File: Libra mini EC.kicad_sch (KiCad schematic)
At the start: 47 parts, among them J1 USB_C_Receptacle_USB2.0_16P, J3 Conn_01x18, J4 Conn_01x18, U1 STM32G474CBTx, U2 USBLC6-2SC6, U3 TPS7A2033, U4 TPS7A2033, U5 TPS7A2033, Y1 8Mhz 12pF

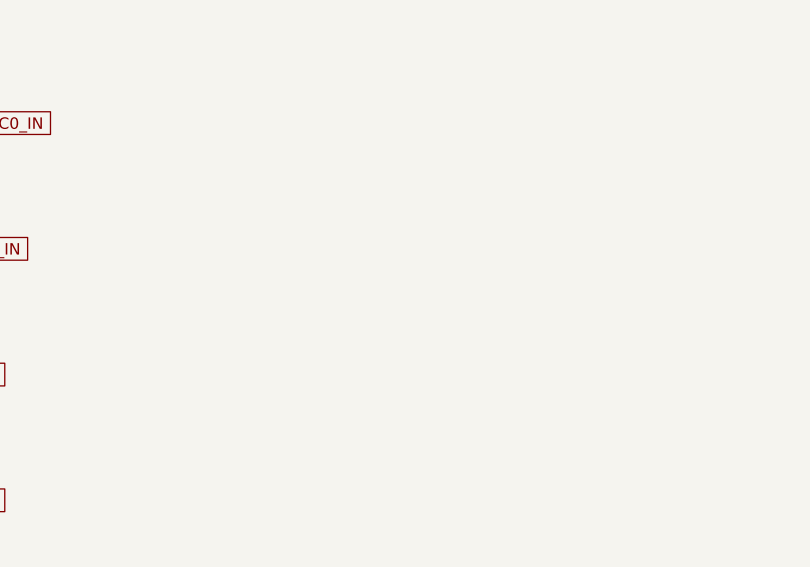
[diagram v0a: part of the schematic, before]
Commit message: 14.04.2026
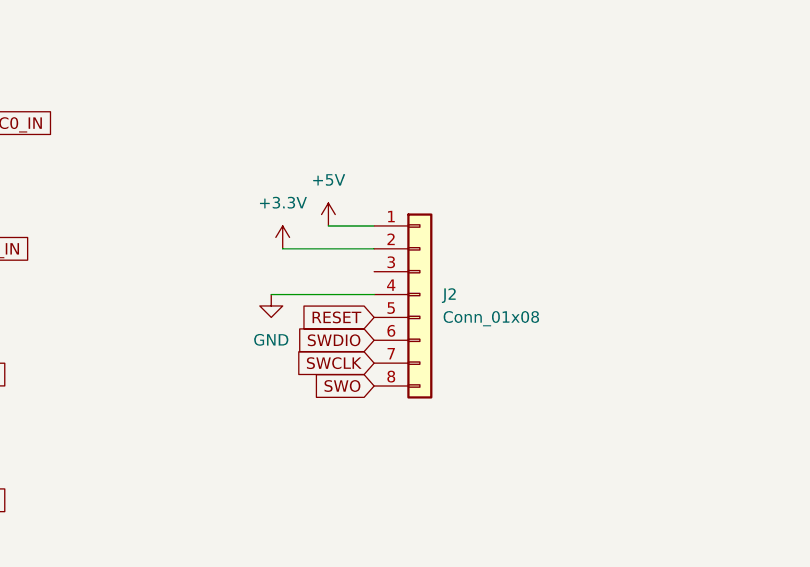
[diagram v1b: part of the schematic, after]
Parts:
- added J2: Conn_01x08, Kicad footprints:SOICbite_footprint, symbol Connector_Generic:Conn_01x08
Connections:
- net +3.3V: now also J2.2 (Pin_2)
- net +5V: now also J2.1 (Pin_1)
- net GND: now also J2.4 (Pin_4)
- net RESET: now also J2.5 (Pin_5)
- new net SWCLK: J2.7 (Pin_7)
- new net SWDIO: J2.6 (Pin_6)
- new net SWO: J2.8 (Pin_8)
